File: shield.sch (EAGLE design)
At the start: 40 parts, among them IC1 AD623R, IC2 AD623R, IC3 AD623R

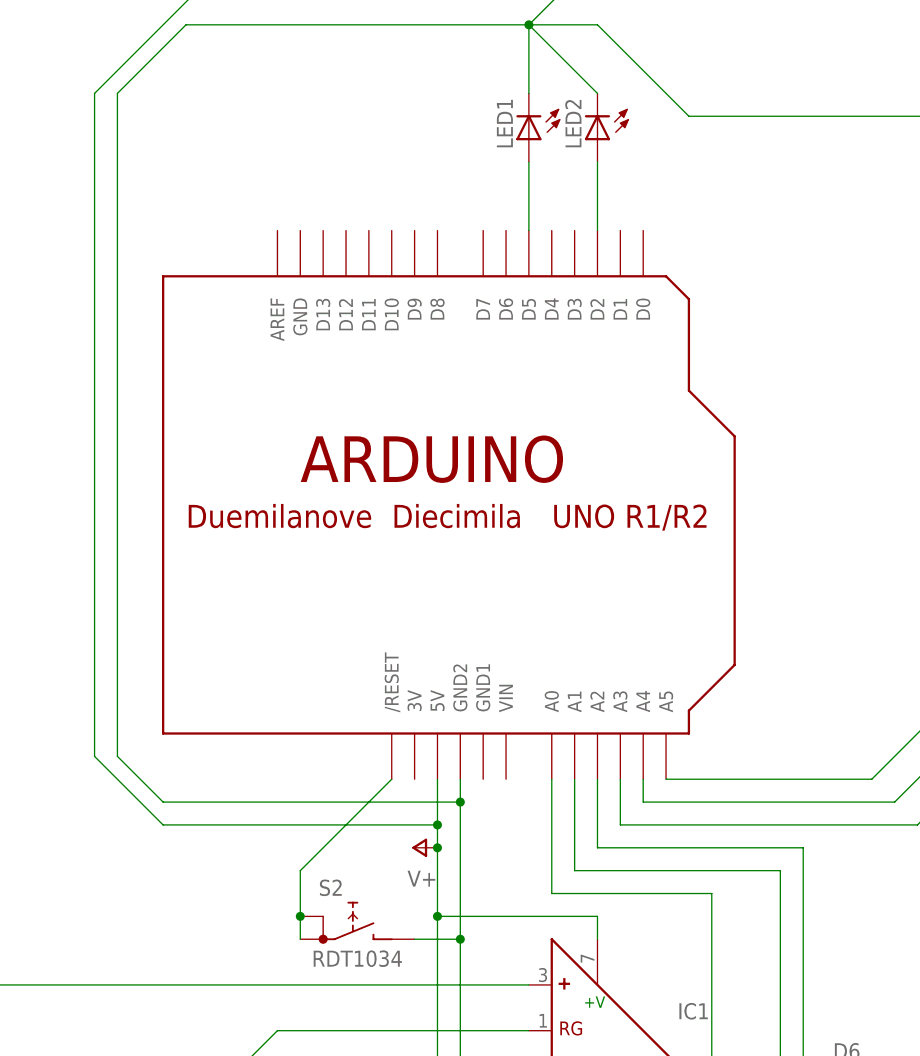
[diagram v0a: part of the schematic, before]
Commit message: Fixed more errors
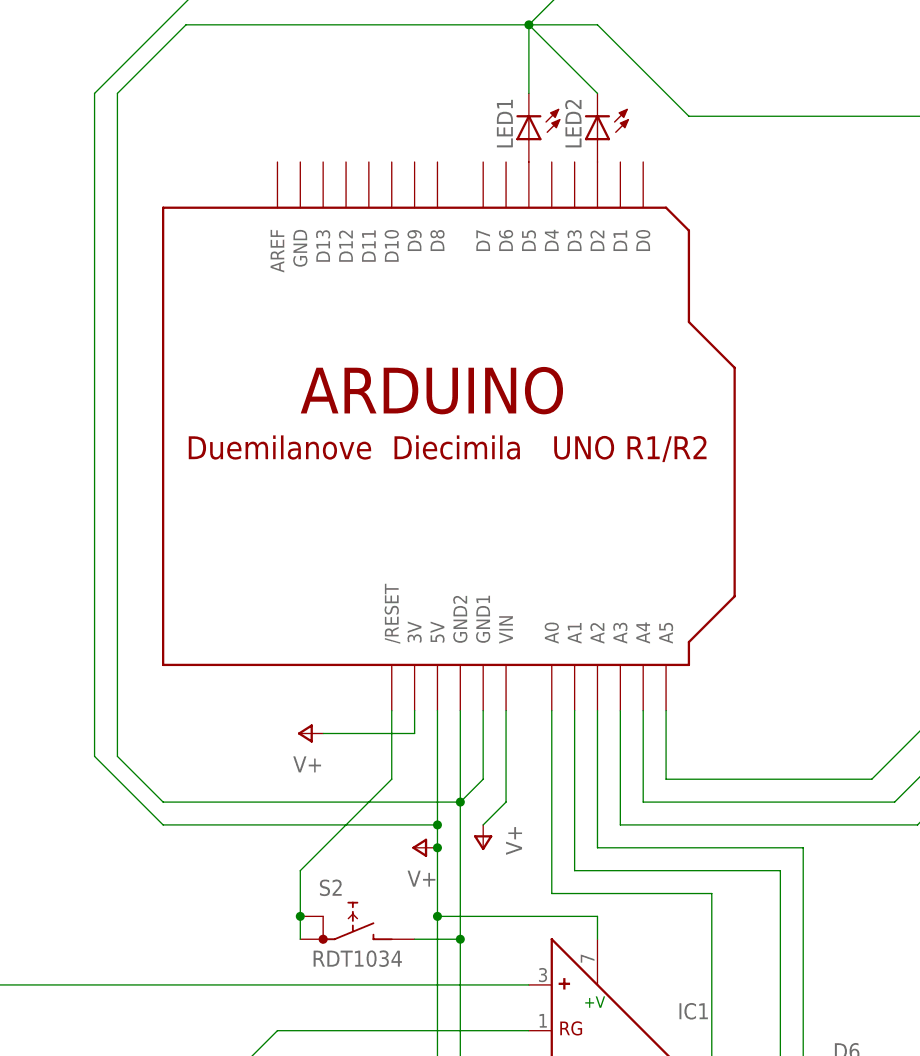
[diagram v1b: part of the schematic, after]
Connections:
- net GND: now also U$1.GND1
- net V+: now also U$1.3V, U$1.VIN
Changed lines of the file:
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@@
 <part name="R25" library="resistor" deviceset="R-EU_" device="0207/10"/>
 <part name="R26" library="resistor" deviceset="R-EU_" device="0207/10"/>
+<part name="P+2" library="supply1" deviceset="V+" device=""/>
+<part name="P+3" library="supply1" deviceset="V+" device=""/>
 </parts>
 <sheets>
@@
 <instance part="IC2" gate="G$1" x="-60.96" y="-63.5"/>
 <instance part="IC3" gate="G$1" x="-60.96" y="-109.22"/>
-<instance part="U$1" gate="G$1" x="-86.36" y="40.64"/>
+<instance part="U$1" gate="G$1" x="-86.36" y="48.26"/>
 <instance part="S2" gate="G$1" x="-88.9" y="-7.62"/>
 <instance part="S1" gate="G$1" x="-114.3" y="-73.66"/>
@@
 <instance part="R25" gate="G$1" x="48.26" y="109.22" rot="R270"/>
 <instance part="R26" gate="G$1" x="25.4" y="99.06" rot="R90"/>
+<instance part="P+2" gate="1" x="-93.98" y="12.7" rot="R90"/>
+<instance part="P+3" gate="1" x="-73.66" y="0" rot="R180"/>
 </instances>
 <busses>
@@
 <segment>
 <pinref part="U$1" gate="G$1" pin="A0"/>
-<wire x1="-66.04" y1="7.62" x2="-66.04" y2="-5.08" width="0.1524" layer="91"/>
+<wire x1="-66.04" y1="15.24" x2="-66.04" y2="-5.08" width="0.1524" layer="91"/>
 <pinref part="IC1" gate="G$1" pin="OUT"/>
 <wire x1="-66.04" y1="-5.08" x2="-48.26" y2="-5.08" width="0.1524" layer="91"/>
@@
 <segment>
 <pinref part="U$1" gate="G$1" pin="A1"/>
-<wire x1="-63.5" y1="7.62" x2="-63.5" y2="-2.54" width="0.1524" layer="91"/>
+<wire x1="-63.5" y1="15.24" x2="-63.5" y2="-2.54" width="0.1524" layer="91"/>
 <wire x1="-63.5" y1="-2.54" x2="-40.64" y2="-2.54" width="0.1524" layer="91"/>
 <wire x1="-40.64" y1="-2.54" x2="-40.64" y2="-63.5" width="0.1524" layer="91"/>
@@
 <segment>
 <pinref part="U$1" gate="G$1" pin="A2"/>
-<wire x1="-60.96" y1="7.62" x2="-60.96" y2="0" width="0.1524" layer="91"/>
+<wire x1="-60.96" y1="15.24" x2="-60.96" y2="0" width="0.1524" layer="91"/>
 <wire x1="-60.96" y1="0" x2="-38.1" y2="0" width="0.1524" layer="91"/>
 <wire x1="-38.1" y1="0" x2="-38.1" y2="-109.22" width="0.1524" layer="91"/>
@@
 <segment>
 <pinref part="U$1" gate="G$1" pin="A3"/>
-<wire x1="-58.42" y1="7.62" x2="-58.42" y2="2.54" width="0.1524" layer="91"/>
+<wire x1="-58.42" y1="15.24" x2="-58.42" y2="2.54" width="0.1524" layer="91"/>
 <wire x1="-58.42" y1="2.54" x2="-25.4" y2="2.54" width="0.1524" layer="91"/>
 <wire x1="-25.4" y1="2.54" x2="2.54" y2="30.48" width="0.1524" layer="91"/>
@@
 <segment>
 <pinref part="U$1" gate="G$1" pin="A4"/>
-<wire x1="-55.88" y1="7.62" x2="-55.88" y2="5.08" width="0.1524" layer="91"/>
+<wire x1="-55.88" y1="15.24" x2="-55.88" y2="5.08" width="0.1524" layer="91"/>
 <wire x1="-55.88" y1="5.08" x2="-27.94" y2="5.08" width="0.1524" layer="91"/>
 <wire x1="-27.94" y1="5.08" x2="17.78" y2="50.8" width="0.1524" layer="91"/>
@@
 <segment>
 <pinref part="U$1" gate="G$1" pin="A5"/>
+<wire x1="-53.34" y1="15.24" x2="-53.34" y2="7.62" width="0.1524" layer="91"/>
 <wire x1="-53.34" y1="7.62" x2="-30.48" y2="7.62" width="0.1524" layer="91"/>
 <wire x1="-30.48" y1="7.62" x2="33.02" y2="71.12" width="0.1524" layer="91"/>
@@
 <net name="N$19" class="0">
 <segment>
-<pinref part="U$1" gate="G$1" pin="/RESET"/>
-<wire x1="-83.82" y1="7.62" x2="-93.98" y2="-2.54" width="0.1524" layer="91"/>
 <pinref part="S2" gate="G$1" pin="A1"/>
 <wire x1="-93.98" y1="-2.54" x2="-93.98" y2="-7.62" width="0.1524" layer="91"/>
@@
 <wire x1="-93.98" y1="-7.62" x2="-93.98" y2="-10.16" width="0.1524" layer="91"/>
 <junction x="-93.98" y="-7.62"/>
+<pinref part="U$1" gate="G$1" pin="/RESET"/>
+<wire x1="-83.82" y1="15.24" x2="-83.82" y2="7.62" width="0.1524" layer="91"/>
+<wire x1="-83.82" y1="7.62" x2="-93.98" y2="-2.54" width="0.1524" layer="91"/>
 </segment>
 </net>
@@
 <pinref part="LED2" gate="G$1" pin="A"/>
 <pinref part="U$1" gate="G$1" pin="D2"/>
-<wire x1="-60.96" y1="76.2" x2="-60.96" y2="68.58" width="0.1524" layer="91"/>
 </segment>
 </net>
@@
 <pinref part="LED1" gate="G$1" pin="A"/>
 <pinref part="U$1" gate="G$1" pin="D5"/>
-<wire x1="-68.58" y1="76.2" x2="-68.58" y2="68.58" width="0.1524" layer="91"/>
 </segment>
 </net>
@@
 <junction x="-60.96" y="-127"/>
 <pinref part="U$1" gate="G$1" pin="GND2"/>
-<wire x1="-76.2" y1="7.62" x2="-76.2" y2="5.08" width="0.1524" layer="91"/>
+<wire x1="-76.2" y1="15.24" x2="-76.2" y2="5.08" width="0.1524" layer="91"/>
 <pinref part="S2" gate="G$1" pin="B"/>
 <wire x1="-76.2" y1="5.08" x2="-76.2" y2="-10.16" width="0.1524" layer="91"/>
@@
 <junction x="78.74" y="60.96"/>
 <junction x="50.8" y="81.28"/>
+<pinref part="U$1" gate="G$1" pin="GND1"/>
+<wire x1="-73.66" y1="15.24" x2="-73.66" y2="7.62" width="0.1524" layer="91"/>
+<wire x1="-73.66" y1="7.62" x2="-76.2" y2="5.08" width="0.1524" layer="91"/>
 </segment>
 </net>
@@
 <wire x1="-78.74" y1="-7.62" x2="-78.74" y2="-45.72" width="0.1524" layer="91"/>
 <wire x1="-78.74" y1="-45.72" x2="-78.74" y2="-91.44" width="0.1524" layer="91"/>
-<wire x1="-78.74" y1="7.62" x2="-78.74" y2="2.54" width="0.1524" layer="91"/>
+<wire x1="-78.74" y1="15.24" x2="-78.74" y2="2.54" width="0.1524" layer="91"/>
 <wire x1="-78.74" y1="2.54" x2="-78.74" y2="0" width="0.1524" layer="91"/>
 <wire x1="-78.74" y1="0" x2="-78.74" y2="-7.62" width="0.1524" layer="91"/>
@@
 <wire x1="-30.48" y1="170.18" x2="-116.84" y2="83.82" width="0.1524" layer="91"/>
 </segment>
-</net>
+<segment>
+<pinref part="U$1" gate="G$1" pin="3V"/>
+<pinref part="P+2" gate="1" pin="V+"/>
+<wire x1="-81.28" y1="15.24" x2="-81.28" y2="12.7" width="0.1524" layer="91"/>
+<wire x1="-81.28" y1="12.7" x2="-91.44" y2="12.7" width="0.1524" layer="91"/>
+</segment>
+<segment>
+<pinref part="P+3" gate="1" pin="V+"/>
+<pinref part="U$1" gate="G$1" pin="VIN"/>
+<wire x1="-73.66" y1="2.54" x2="-71.12" y2="5.08" width="0.1524" layer="91"/>
+<wire x1="-71.12" y1="5.08" x2="-71.12" y2="15.24" width="0.1524" layer="91"/>
+</segment>
+</net>
